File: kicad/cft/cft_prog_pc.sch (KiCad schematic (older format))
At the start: 23 parts, among them U501 74HCT541, U502 74HC193, U503 74HC541, U504 74HCT541, U505 74HC193, U506 74HCT541, U507 74HC193, U508 74HC541, U509 74HCT541, U510 74HC193, U511 74HC541

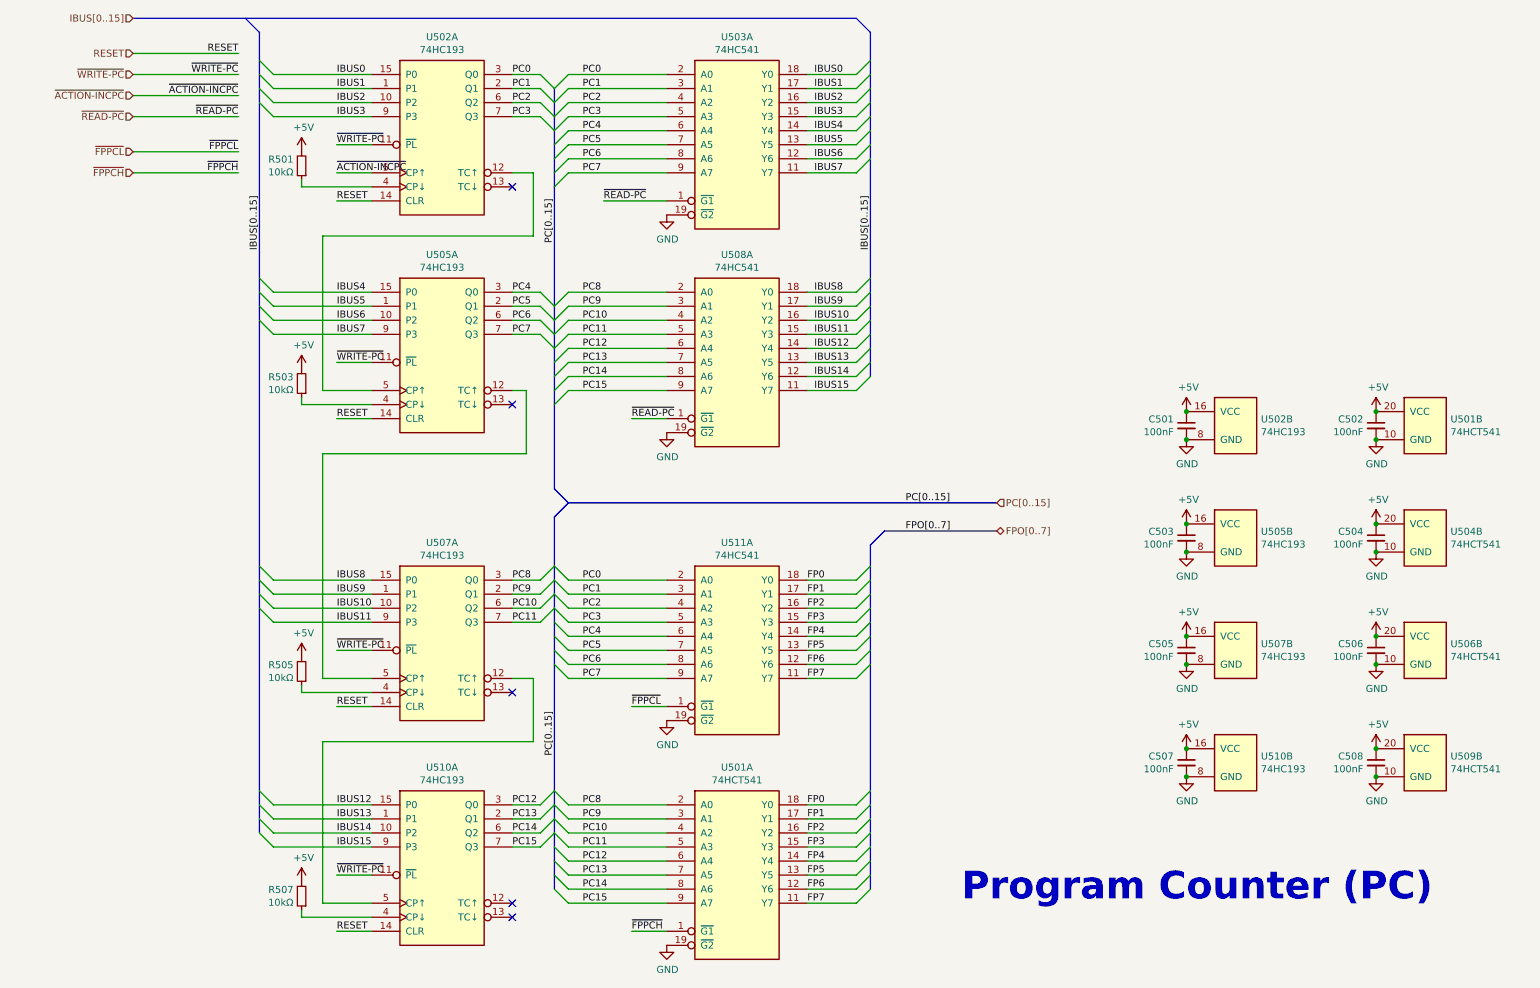
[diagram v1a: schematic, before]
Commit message: Moved things around a bit
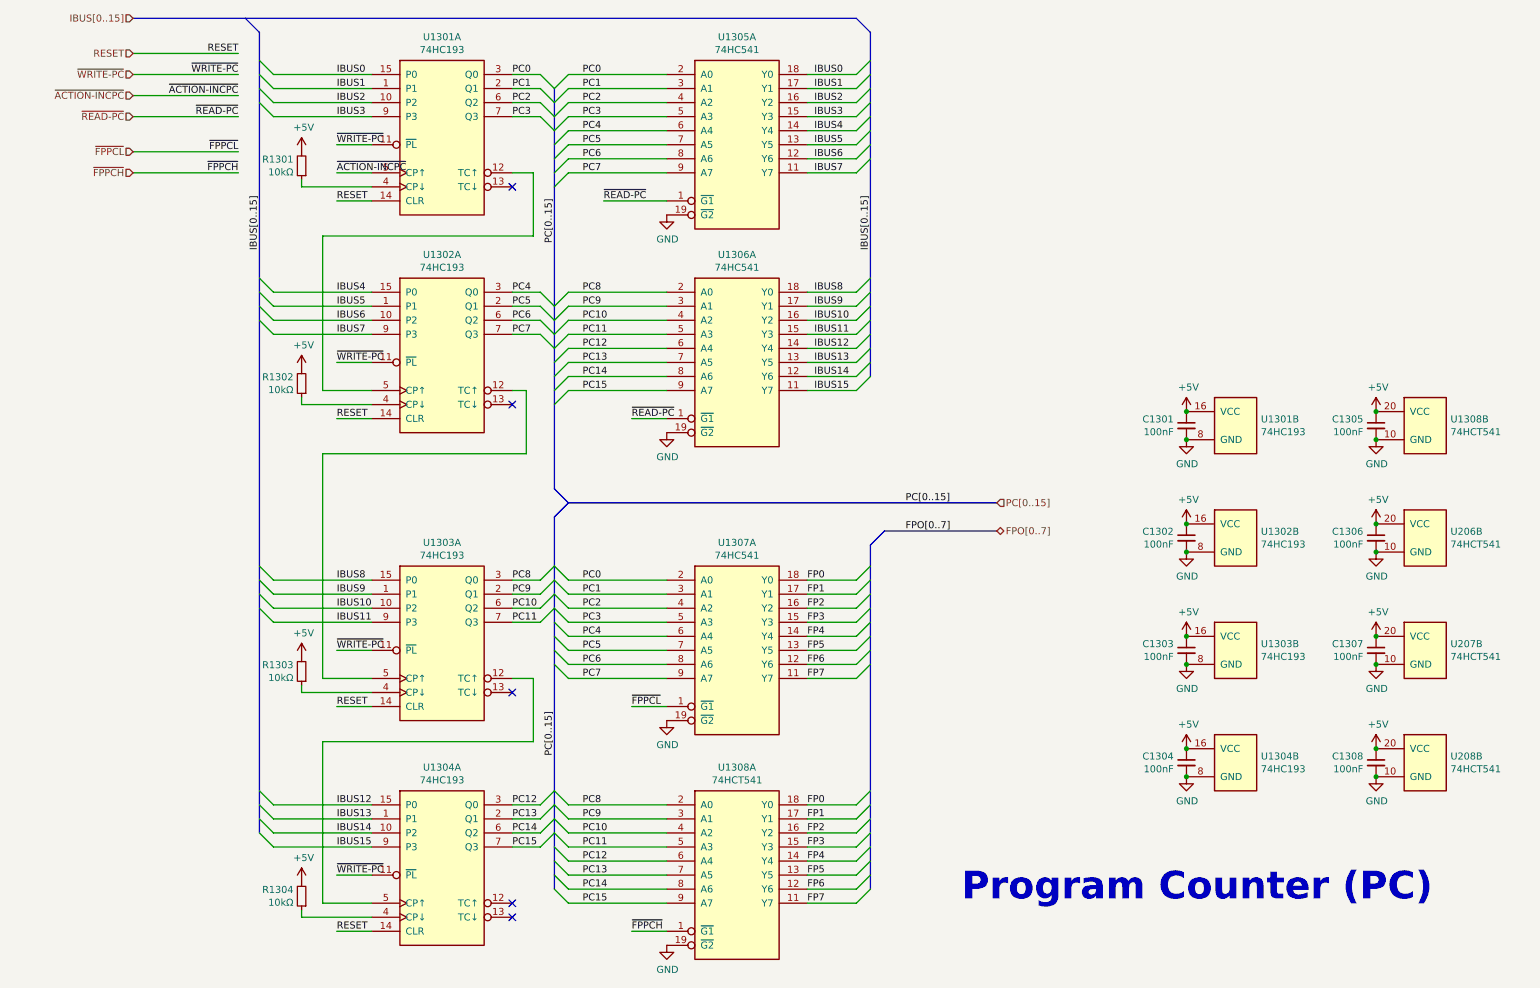
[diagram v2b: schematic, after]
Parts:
- renumbered C501 to C1301, C503 to C1302, C505 to C1303, C507 to C1304, C502 to C1305, C504 to C1306, C506 to C1307, C508 to C1308, R501 to R1301, R503 to R1302, R505 to R1303, R507 to R1304, U502 to U1301, U505 to U1302, U507 to U1303, U510 to U1304, U503 to U1305, U508 to U1306, U511 to U1307, U501 to U1308, U504 to U206, U506 to U207, U509 to U208

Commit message: Removed widebus buffer from microcode store µAddr High
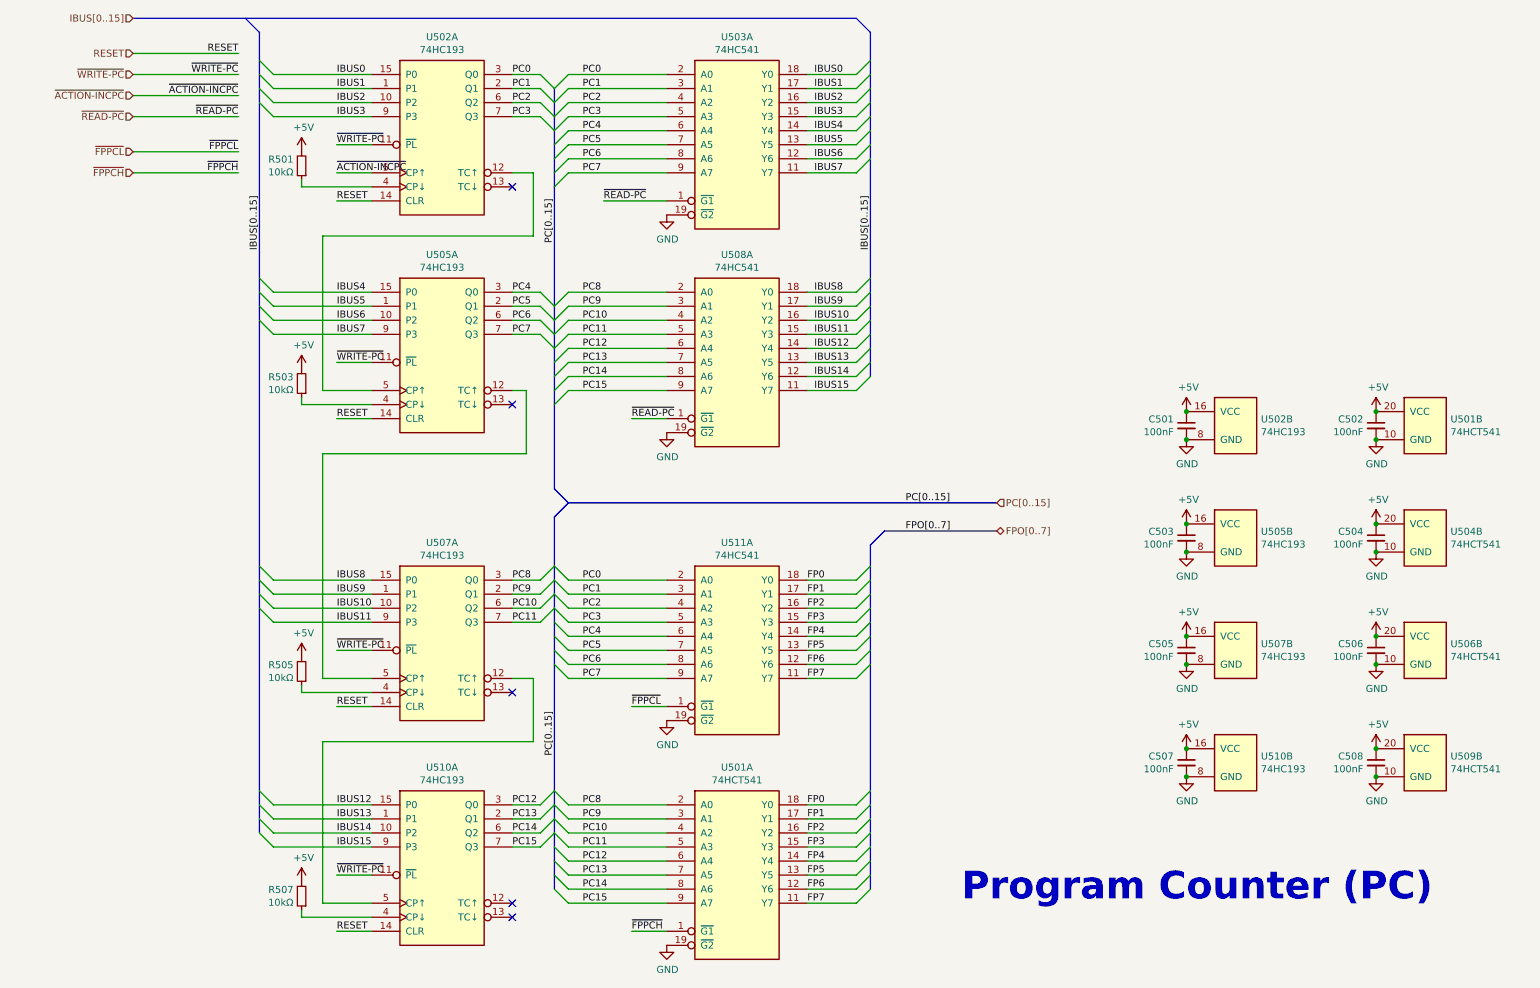
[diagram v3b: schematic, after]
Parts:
- renumbered C1301 to C501, C1305 to C502, C1302 to C503, C1306 to C504, C1303 to C505, C1307 to C506, C1304 to C507, C1308 to C508, R1301 to R501, R1302 to R503, R1303 to R505, R1304 to R507, U1308 to U501, U1301 to U502, U1305 to U503, U206 to U504, U1302 to U505, U207 to U506, U1303 to U507, U1306 to U508, U208 to U509, U1304 to U510, U1307 to U511
